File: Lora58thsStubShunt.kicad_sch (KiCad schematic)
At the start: 11 parts, among them J1 Conn_Coaxial, J2 Conn_01x01_Pin, J3 Conn_01x01_Pin, J4 Conn_01x01_Pin

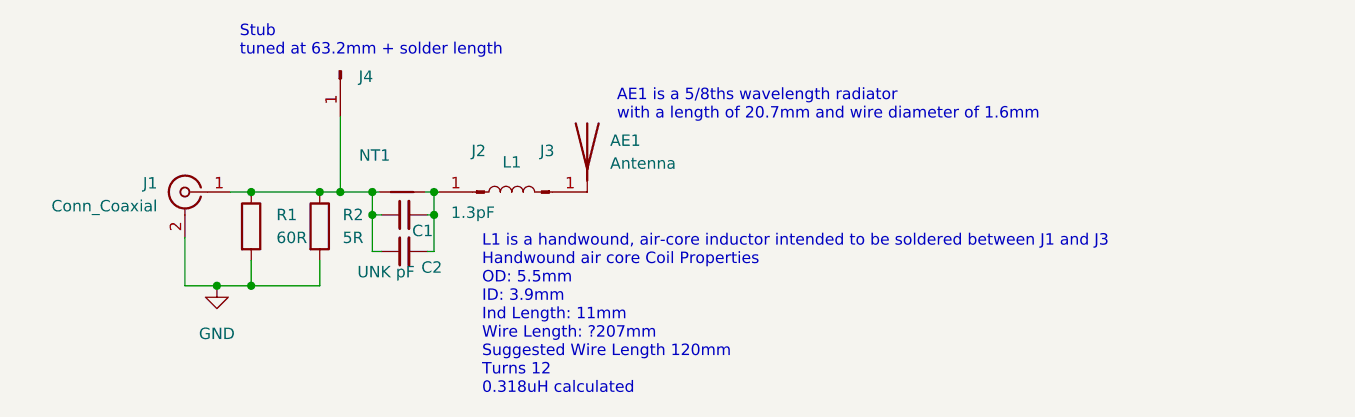
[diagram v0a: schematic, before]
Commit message: Release Candidate
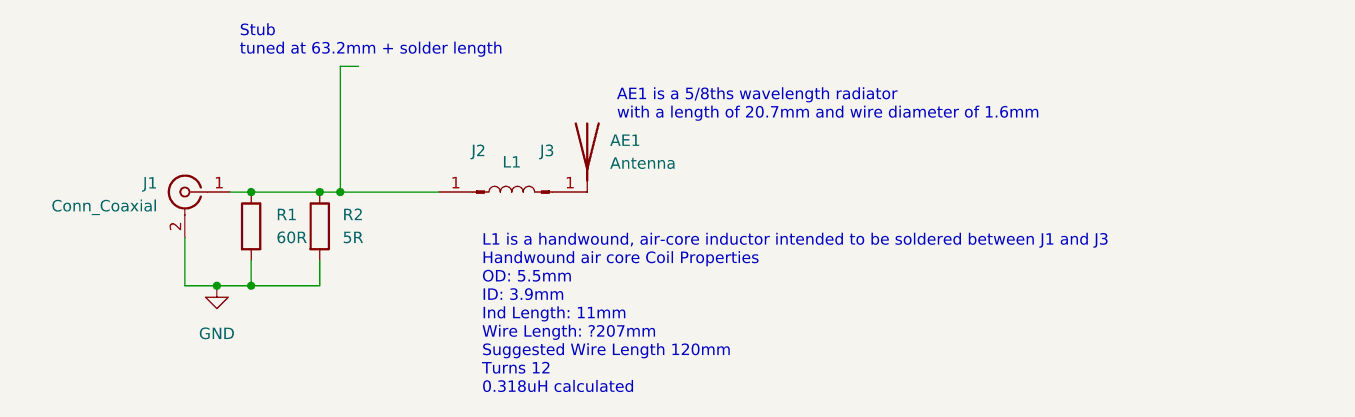
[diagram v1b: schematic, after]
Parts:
- removed C1: 1.3pF, Resistor_SMD:R_0402_1005Metric_Pad0.72x0.64mm_HandSolder, symbol Device:C_Small
- removed C2: UNK pF, Resistor_SMD:R_0402_1005Metric_Pad0.72x0.64mm_HandSolder, symbol Device:C_Small
- removed J4: Conn_01x01_Pin, TestPoint:TestPoint_Keystone_5015_Micro-Minature, symbol Connector:Conn_01x01_Pin
- removed NT1: NetTie_2, Jumper:SolderJumper-2_P1.3mm_Open_RoundedPad1.0x1.5mm, symbol Device:NetTie_2
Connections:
- net at J1.1 (In), R1.1, R2.1: now also J2.1 (Pin_1)
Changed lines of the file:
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@@
   (junction (at 64.008 78.232) (diameter 0) (color 0 0 0 0)
-  )
-  (junction (at 74.422 78.232) (diameter 0) (color 0 0 0 0)
   )
   (junction (at 54.102 78.232) (diameter 0) (color 0 0 0 0)
   )
-  (junction (at 67.564 80.772) (diameter 0) (color 0 0 0 0)
-  )
   (junction (at 61.722 78.232) (diameter 0) (color 0 0 0 0)
-  )
-  (junction (at 74.422 80.772) (diameter 0) (color 0 0 0 0)
-  )
-  (junction (at 67.564 78.232) (diameter 0) (color 0 0 0 0)
   )
   (junction (at 54.102 88.646) (diameter 0) (color 0 0 0 0)
   )
-  (wire (pts (xy 64.008 69.85) (xy 64.008 78.232))
-    (stroke (width 0) (type default))
-  )
-  (wire (pts (xy 67.564 80.772) (xy 67.564 84.836))
-    (stroke (width 0) (type default))
-  )
-  (wire (pts (xy 73.406 78.232) (xy 74.422 78.232))
-    (stroke (width 0) (type default))
-  )
-  (wire (pts (xy 68.58 84.836) (xy 67.564 84.836))
-    (stroke (width 0) (type default))
-  )
-  (wire (pts (xy 67.564 78.232) (xy 68.326 78.232))
+  (wire (pts (xy 64.008 64.262) (xy 64.008 78.232))
     (stroke (width 0) (type default))
   )
@@
     (stroke (width 0) (type default))
   )
-  (wire (pts (xy 74.422 78.232) (xy 74.422 80.772))
-    (stroke (width 0) (type default))
-  )
   (wire (pts (xy 51.816 78.232) (xy 54.102 78.232))
-    (stroke (width 0) (type default))
-  )
-  (wire (pts (xy 68.58 80.772) (xy 67.564 80.772))
     (stroke (width 0) (type default))
   )
@@
     (stroke (width 0) (type default))
   )
-  (wire (pts (xy 74.422 78.232) (xy 74.93 78.232))
-    (stroke (width 0) (type default))
-  )
-  (wire (pts (xy 67.564 77.978) (xy 67.564 78.232))
-    (stroke (width 0) (type default))
-  )
-  (wire (pts (xy 73.66 84.836) (xy 74.422 84.836))
-    (stroke (width 0) (type default))
-  )
-  (wire (pts (xy 73.66 80.772) (xy 74.422 80.772))
-    (stroke (width 0) (type default))
-  )
-  (wire (pts (xy 64.008 78.232) (xy 67.564 78.232))
-    (stroke (width 0) (type default))
-  )
-  (wire (pts (xy 74.422 80.772) (xy 74.422 84.836))
+  (wire (pts (xy 64.008 78.232) (xy 74.93 78.232))
     (stroke (width 0) (type default))
   )
   (wire (pts (xy 61.722 78.232) (xy 64.008 78.232))
-    (stroke (width 0) (type default))
-  )
-  (wire (pts (xy 67.564 78.232) (xy 67.564 80.772))
     (stroke (width 0) (type default))
   )
@@
     (stroke (width 0) (type default))
   )
+  (wire (pts (xy 64.008 64.262) (xy 66.04 64.262))
+    (stroke (width 0) (type default))
+  )
   (text "AE1 is a 5/8ths wavelength radiator \nwith a length of 20.7mm and wire diameter of 1.6mm"
     (at 94.742 70.358 0)
@@
     (at 79.756 100.838 0)
     (effects (font (size 1.27 1.27)) (justify left bottom))
-  )
-  (symbol (lib_id "Device:NetTie_2") (at 70.866 78.232 0) (unit 1)
-    (in_bom no) (on_board yes) (dnp no)
-    (property "Reference" "NT1" (at 67.818 74.168 0)
-      (effects (font (size 1.27 1.27)))
-    )
-    (property "Value" "NetTie_2" (at 70.866 76.2 0)
-      (effects (font (size 1.27 1.27)) hide)
-    )
-    (property "Footprint" "Jumper:SolderJumper-2_P1.3mm_Open_RoundedPad1.0x1.5mm" (at 70.866 78.232 0)
-      (effects (font (size 1.27 1.27)) hide)
-    )
-    (property "Datasheet" "~" (at 70.866 78.232 0)
-      (effects (font (size 1.27 1.27)) hide)
-    )
-    (pin "1")
-    (pin "2")
-    (instances
-      (project "Lora58thsStubShunt"
-        (path "/cf900f9d-35df-470e-ae2b-7ec23d8c16cd"
-          (reference "NT1") (unit 1)
-        )
-      )
-    )
   )
   (symbol (lib_id "Device:Antenna") (at 91.44 73.152 0) (unit 1)
@@
         (path "/cf900f9d-35df-470e-ae2b-7ec23d8c16cd"
           (reference "R2") (unit 1)
-        )
-      )
-    )
-  )
-  (symbol (lib_id "Device:C_Small") (at 71.12 84.836 90) (unit 1)
-    (in_bom yes) (on_board yes) (dnp no)
-    (property "Reference" "C2" (at 74.168 86.614 90)
-      (effects (font (size 1.27 1.27)))
-    )
-    (property "Value" "UNK pF" (at 69.088 87.122 90)
-      (effects (font (size 1.27 1.27)))
-    )
-    (property "Footprint" "Resistor_SMD:R_0402_1005Metric_Pad0.72x0.64mm_HandSolder" (at 71.12 84.836 0)
-      (effects (font (size 1.27 1.27)) hide)
-    )
-    (property "Datasheet" "~" (at 71.12 84.836 0)
-      (effects (font (size 1.27 1.27)) hide)
-    )
-    (pin "1")
-    (pin "2")
-    (instances
-      (project "Lora58thsStubShunt"
-        (path "/cf900f9d-35df-470e-ae2b-7ec23d8c16cd"
-          (reference "C2") (unit 1)
         )
       )
@@
         )
       )
-    )
-  )
-  (symbol (lib_id "Device:C_Small") (at 71.12 80.772 90) (unit 1)
-    (in_bom yes) (on_board yes) (dnp no)
-    (property "Reference" "C1" (at 73.152 82.55 90)
-      (effects (font (size 1.27 1.27)))
-    )
-    (property "Value" "1.3pF" (at 78.74 80.518 90)
-      (effects (font (size 1.27 1.27)))
-    )
-    (property "Footprint" "Resistor_SMD:R_0402_1005Metric_Pad0.72x0.64mm_HandSolder" (at 71.12 80.772 0)
-      (effects (font (size 1.27 1.27)) hide)
-    )
-    (property "Datasheet" "~" (at 71.12 80.772 0)
-      (effects (font (size 1.27 1.27)) hide)
-    )
-    (pin "1")
-    (pin "2")
-    (instances
-      (project "Lora58thsStubShunt"
-        (path "/cf900f9d-35df-470e-ae2b-7ec23d8c16cd"
-          (reference "C1") (unit 1)
-        )
-      )
-    )
-  )
-  (symbol (lib_id "Connector:Conn_01x01_Pin") (at 64.008 64.77 90) (mirror x) (unit 1)
-    (in_bom yes) (on_board yes) (dnp no) (fields_autoplaced)
-    (property "Reference" "J4" (at 66.04 65.405 90)
-      (effects (font (size 1.27 1.27)) (justify right))
-    )
-    (property "Value" "Conn_01x01_Pin" (at 65.024 66.675 90)
-      (effects (font (size 1.27 1.27)) (justify right) hide)
-    )
-    (property "Footprint" "TestPoint:TestPoint_Keystone_5015_Micro-Minature" (at 64.008 64.77 0)
-      (effects (font (size 1.27 1.27)) hide)
-    )
-    (property "Datasheet" "~" (at 64.008 64.77 0)
-      (effects (font (size 1.27 1.27)) hide)
-    )
-    (pin "1")
-    (instances
-      (project "Lora58thsStubShunt"
-        (path "/cf900f9d-35df-470e-ae2b-7ec23d8c16cd"
-          (reference "J4") (unit 1)
-        )
-      )
